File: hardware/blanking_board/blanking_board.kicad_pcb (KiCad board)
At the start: 2 copper layers, 95 x 82 mm, 23 parts, among them J1 B4B-XH-A_LF__SN_, J10 Conn_01x02_Female, J11 DB25_Female_MountingHoles, J12 DB25_Female_MountingHoles, J2 B4B-XH-A_LF__SN_, J3 B4B-XH-A_LF__SN_, J4 B2B-XH-A_LF__SN_, J5 B4B-XH-A_LF__SN_, J6 B4B-XH-A_LF__SN_, J7 B4B-XH-A_LF__SN_, J8 B4B-XH-A_LF__SN_, J9 Conn_01x02_Female, U1 74HC14, U2 74LS08, U3 74LS08, U4 74LS08

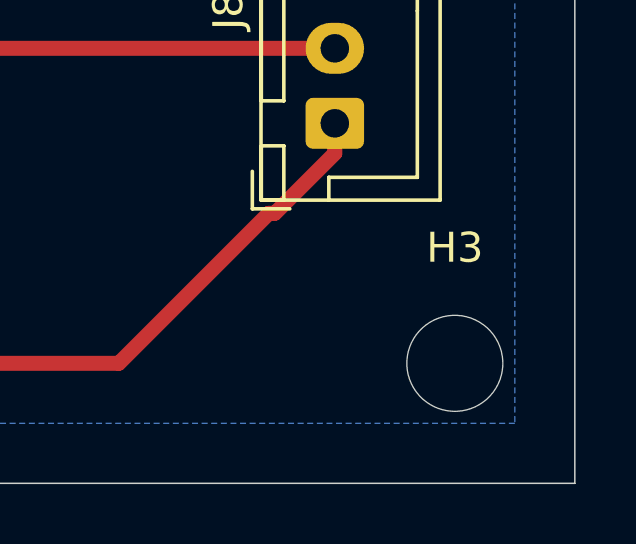
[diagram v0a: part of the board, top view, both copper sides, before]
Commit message: update board details
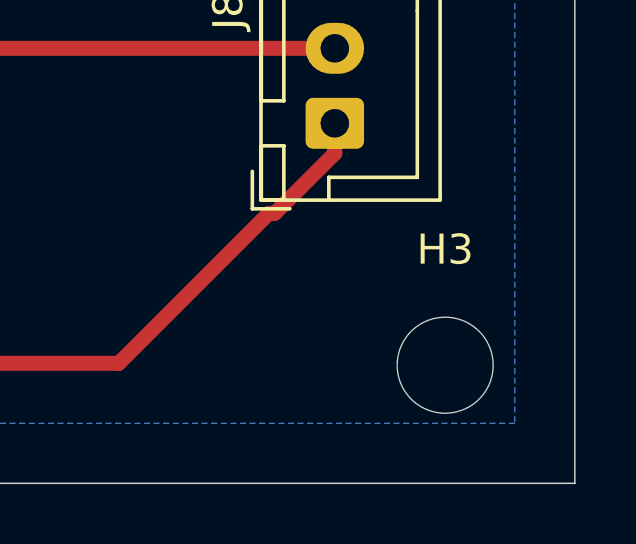
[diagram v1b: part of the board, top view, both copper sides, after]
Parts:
- moved H3 0.33 mm to (188.7, 125.1)
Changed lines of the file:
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@@
   )
   (footprint "MountingHole:MountingHole_3.2mm_M3_ISO7380" (layer "F.Cu")
-    (at 189 125)
+    (at 188.678 125.063)
     (descr "Mounting Hole 3.2mm, no annular, M3, ISO7380")
     (tags "mounting hole 3.2mm no annular m3 iso7380")
@@
       (effects (font (size 1 1) (thickness 0.15)))
     )
-    (fp_text user "${REFERENCE}" (at 0.3 0) (layer "F.Fab")
+    (fp_text user "${REFERENCE}" (at 0.254 0.19) (layer "F.Fab")
       (effects (font (size 1 1) (thickness 0.15)))
     )
@@
       )
     )
+  )
+  (zone (net 0) (net_name "") (layer "B.Cu") (hatch edge 0.508)
+    (connect_pads (clearance 0))
+    (min_thickness 0.254)
+    (keepout (tracks not_allowed) (vias not_allowed) (pads not_allowed ) (copperpour not_allowed) (footprints allowed))
+    (fill (thermal_gap 0.508) (thermal_bridge_width 0.508))
+    (polygon
+      (pts
+        (xy 104.35 53.054)
+        (xy 98.127 53.054)
+        (xy 98.127 47.212)
+        (xy 104.35 47.212)
+      )
+    )
+  )
+  (zone (net 0) (net_name "") (layer "B.Cu") (hatch edge 0.508)
+    (connect_pads (clearance 0))
+    (min_thickness 0.254)
+    (keepout (tracks not_allowed) (vias not_allowed) (pads not_allowed ) (copperpour not_allowed) (footprints allowed))
+    (fill (thermal_gap 0.508) (thermal_bridge_width 0.508))
+    (polygon
+      (pts
+        (xy 190.964 126.968)
+        (xy 184.741 126.968)
+        (xy 184.741 121.126)
+        (xy 190.964 121.126)
+      )
+    )
+  )
+  (zone (net 0) (net_name "") (layer "B.Cu") (hatch edge 0.508)
+    (connect_pads (clearance 0))
+    (min_thickness 0.254)
+    (keepout (tracks not_allowed) (vias not_allowed) (pads not_allowed ) (copperpour not_allowed) (footprints allowed))
+    (fill (thermal_gap 0.508) (thermal_bridge_width 0.508))
+    (polygon
+      (pts
+        (xy 190.964 54.832)
+        (xy 184.741 54.832)
+        (xy 184.741 48.99)
+        (xy 190.964 48.99)
+      )
+    )
+  )
+  (zone (net 0) (net_name "") (layer "B.Cu") (hatch edge 0.508)
+    (connect_pads (clearance 0))
+    (min_thickness 0.254)
+    (keepout (tracks not_allowed) (vias not_allowed) (pads not_allowed ) (copperpour not_allowed) (footprints allowed))
+    (fill (thermal_gap 0.508) (thermal_bridge_width 0.508))
+    (polygon
+      (pts
+        (xy 106.128 126.968)
+        (xy 99.905 126.968)
+        (xy 99.905 121.126)
+        (xy 106.128 121.126)
+      )
+    )
